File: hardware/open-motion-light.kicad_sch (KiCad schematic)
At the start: 99 parts, among them J1 TYPE-C-31-M-12, Q1 2N7002, SW1 SW_Push, SW3 SSSS213800, U1 CN3058E, U2 VCNL4020-GS08, U3 MT9284BS6, U4 XYC-PIR224S-S1, U6 CH340X, U7 STM32L051K8Ux

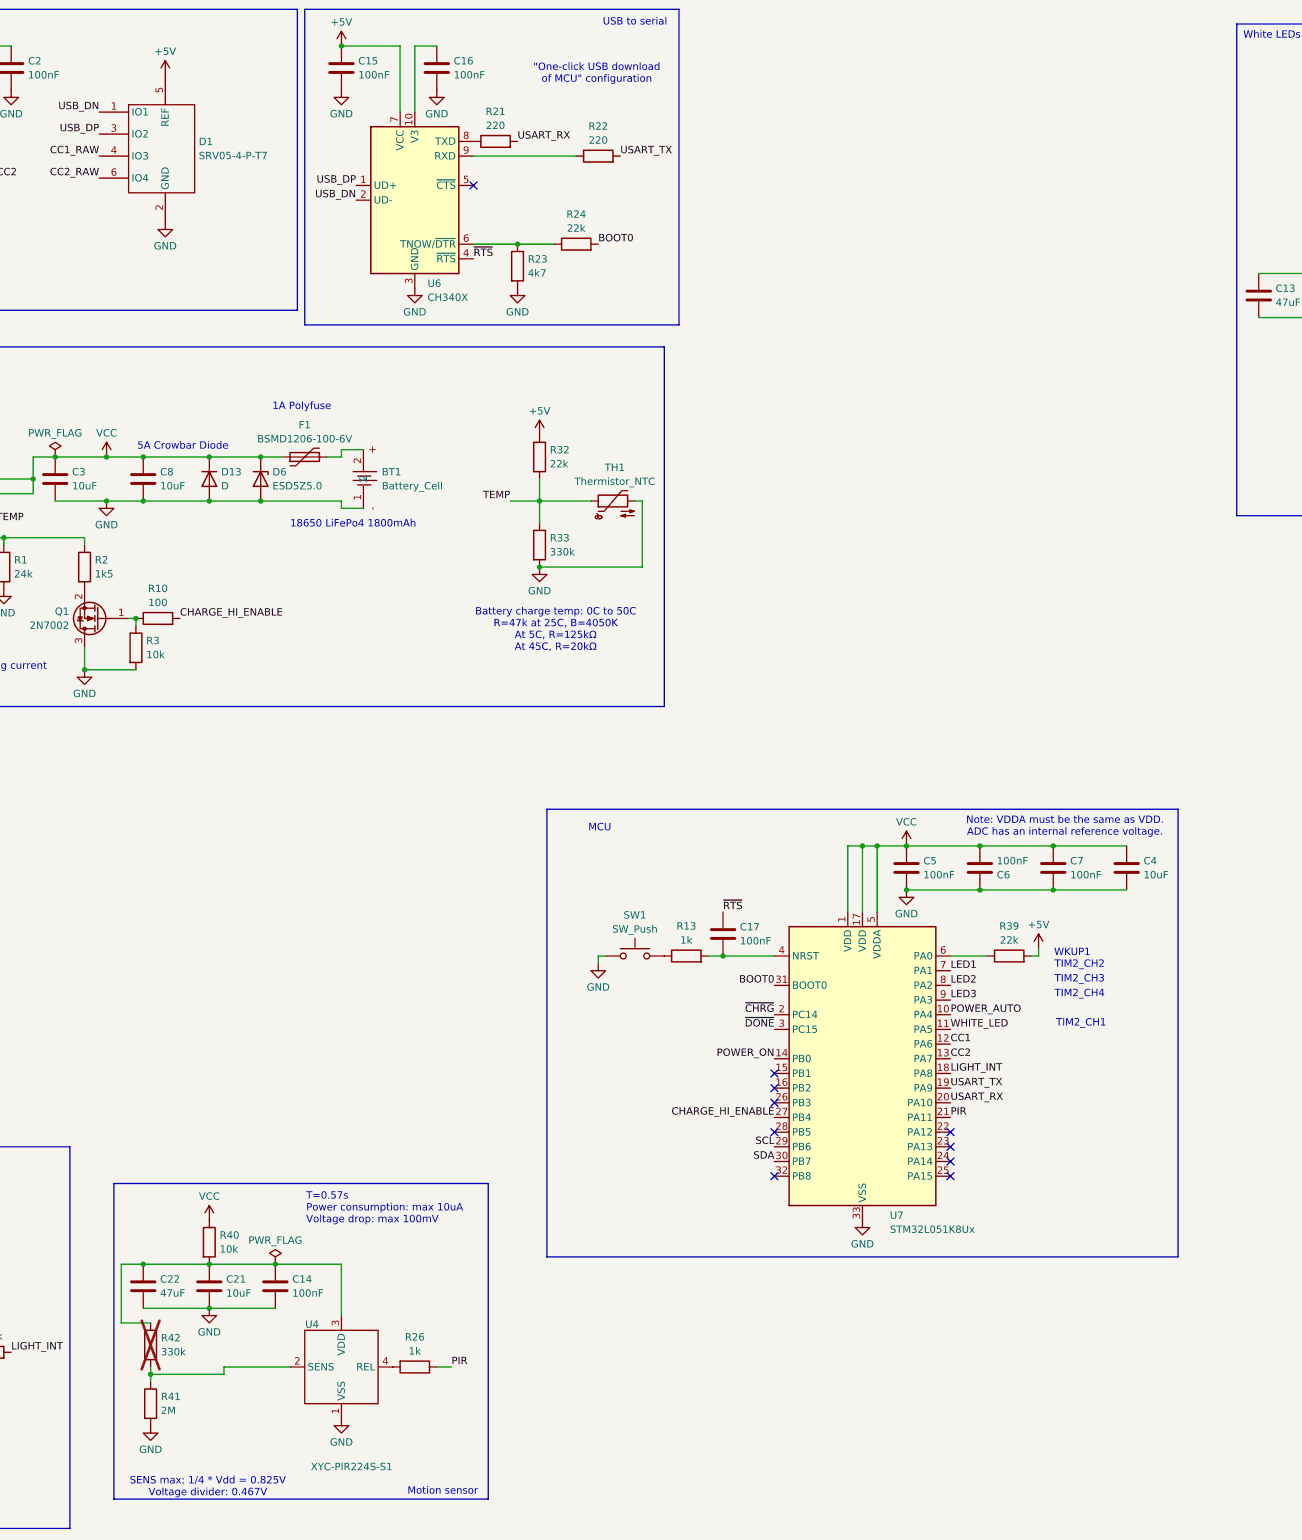
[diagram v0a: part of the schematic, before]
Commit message: Hardware v1.3 first pass
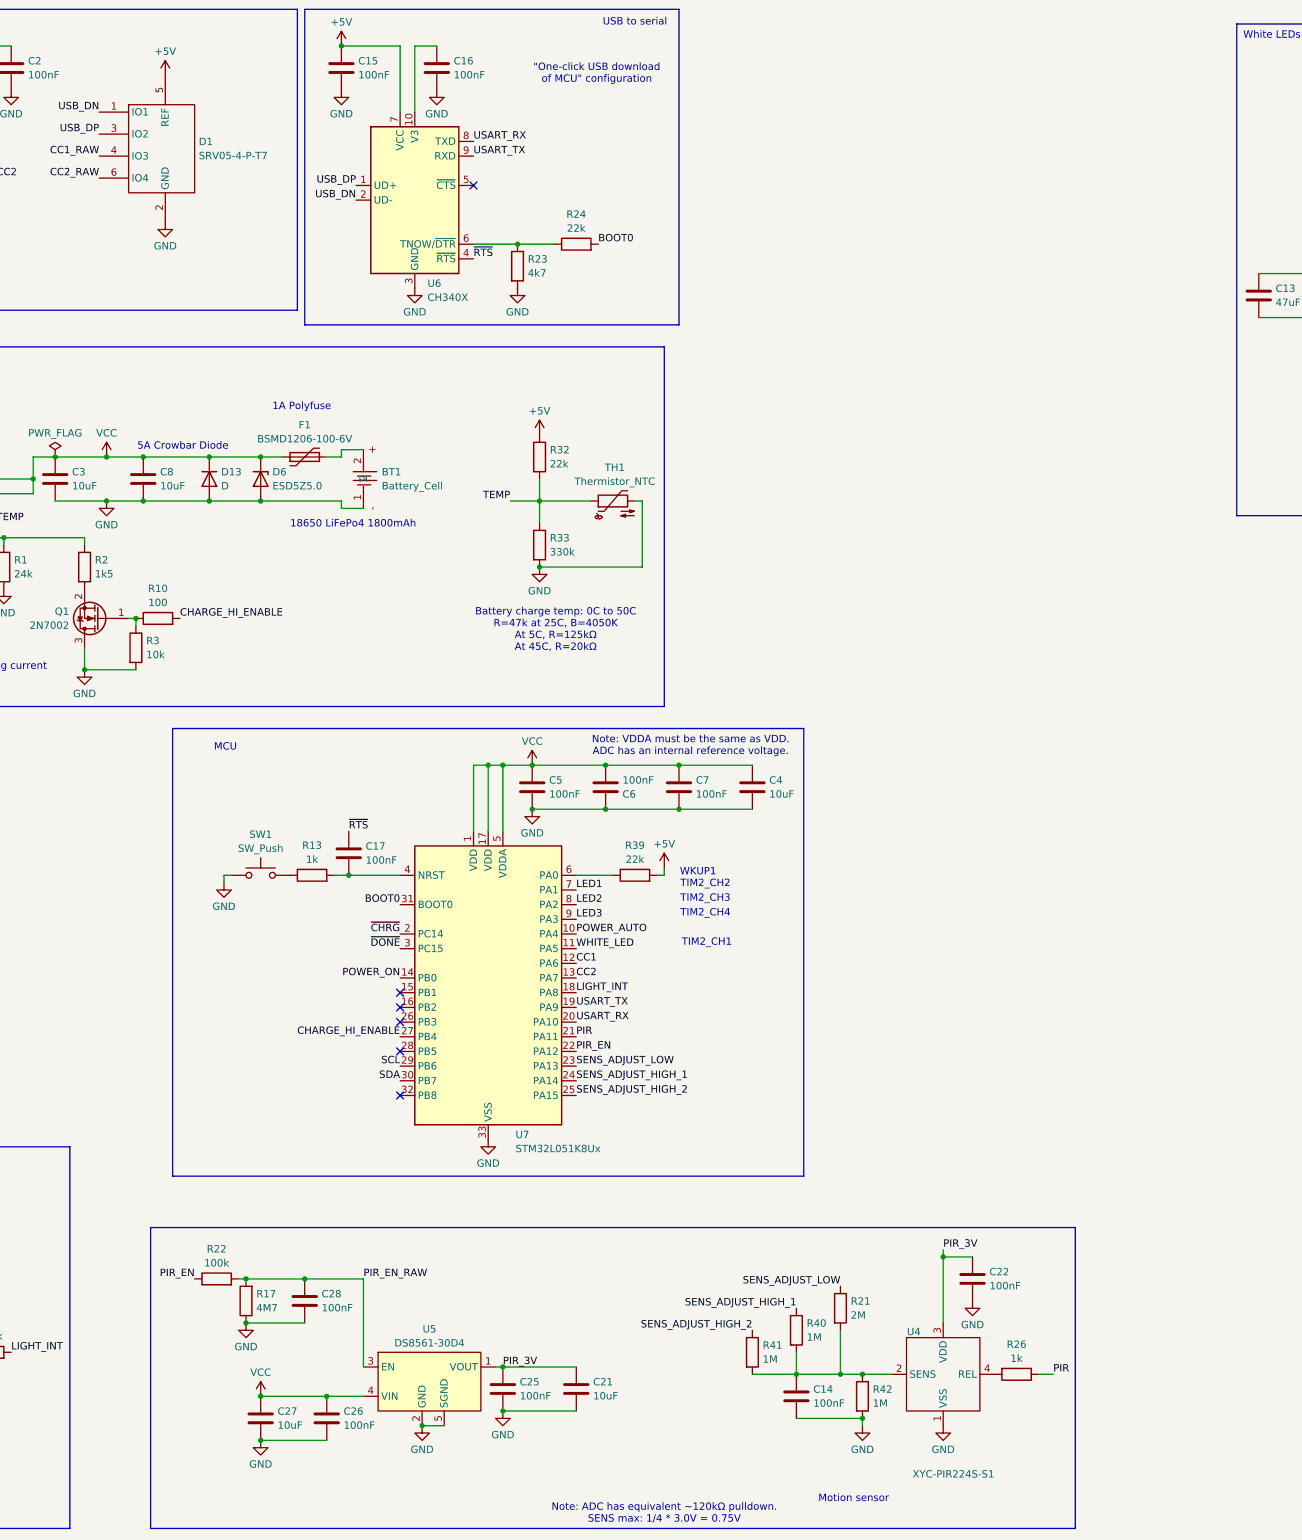
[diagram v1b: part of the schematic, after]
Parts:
- added C25, C26, C28: 100nF, Capacitor_SMD:C_0402_1005Metric, symbol Device:C
- added C27: 10uF, Capacitor_SMD:C_0603_1608Metric, symbol Device:C
- added R17: 4M7, Resistor_SMD:R_0603_1608Metric, symbol Device:R
- added U5: DS8561-30D4, Homebrew:UDFN-4_L1.0-W1.0-P0.65-TL, symbol Homebrew:DS8561-30D4
- C22: value 47uF -> 100nF; footprint Capacitor_SMD:C_1206_3216Metric -> Capacitor_SMD:C_0402_1005Metric; LCSC C96123 -> C307331
- R21: value 220 -> 2M; footprint Resistor_SMD:R_0402_1005Metric -> Resistor_SMD:R_0603_1608Metric; LCSC C25091 -> C422964
- R22: value 220 -> 100k; LCSC C25091 -> C25741
- R40: value 10k -> 1M; footprint Resistor_SMD:R_0603_1608Metric_Pad0.98x0.95mm_HandSolder -> Resistor_SMD:R_0603_1608Metric; LCSC C25804 -> C7250
- R41: value 2M -> 1M; LCSC C22976 -> C7250
- R42: value 330k -> 1M; LCSC C23137 -> C7250; now fitted
- U4: footprint Homebrew:TO-5-4_BD9.2-P2.54_XYC-PIR224D-D0 -> easyeda2kicad:TO-5-4_BD9.2-P2.54_XYC-PIR224D-D0
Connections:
- net GND: now also C22.2, R42.2, C25.2, C26.2, C27.2, C28.2, R17.1, U5.2 (GND), U5.5 (SGND); no longer C22.1, R41.2
- net USART_RX: now also U6.8 (TXD); no longer R21.2
- net USART_TX: now also U6.9 (RXD); no longer R22.2
- net VCC: now also C26.1, C27.1, U5.4 (VIN); no longer R40.1
- net at C14.1, R40.2, R42.1: now also R21.2, R41.2, U4.2 (SENS); no longer C21.1, C22.2, U4.3 (VDD)
- net SENS_ADJUST_LOW: now reaches R21.1
- net SENS_ADJUST_LOW: now also U7.23 (PA13); no longer U6.8 (TXD)
- net PIR_EN: now reaches R22.1
- net PIR_EN: now also U7.22 (PA12); no longer U6.9 (RXD)
- net SENS_ADJUST_HIGH_1: now reaches U7.24 (PA14)
- net SENS_ADJUST_HIGH_1: now also R40.1
- net SENS_ADJUST_HIGH_2: now reaches U7.25 (PA15)
- net SENS_ADJUST_HIGH_2: now also R41.1
- new net PIR_3V: C21.1, C22.1, C25.1, U4.3 (VDD), U5.1 (VOUT)
- new net PIR_EN_RAW: C28.1, R17.2, R22.2, U5.3 (EN)
- no-connect marks 13 -> 9
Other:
- note added: "Note: ADC has equivalent ~120kΩ pulldown. SENS max: 1/4 * 3.0V = 0.75V"
- note removed: "SENS max: 1/4 * Vdd = 0.825V Voltage divider: 0.467V"
- note removed: "T=0.57s Power consumption: max 10uA Voltage drop: max 100mV"
- moved on the sheet: C17, C21, C4, C5, C6, C7, R13, R26, R39, SW1, U4, U7
